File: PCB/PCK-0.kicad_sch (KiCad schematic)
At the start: 102 parts, among them J1 USB_C_Receptacle_USB2.0_16P, J2 BAT+, J3 BAT-, SW1 EN, SW10 5, SW11 M2, SW12 TAB, SW13 Q, SW14 W, SW15 E, SW16 R, SW17 T, SW18 M3, SW19 CAPSLOCK, SW2 BOOT, SW20 A, SW21 S, SW22 D, SW23 F, SW24 G, SW25 M4, SW26 LSHIFT, SW27 Z, SW28 X, SW29 C, SW3 RotaryEncoder_Switch_MP, SW30 V, SW31 SPACE, SW32 M5, SW33 FN, SW34 CTRL, SW35 SUPER, SW36 ALT, SW37 MOD1, SW38 MOD2, SW4 M1, SW5 ESC, SW6 1, SW7 2, SW8 3, SW9 4, U1 NCP1117-3.3_SOT223, U2 NCP1117-3.3_SOT223, U3 USBLC6-2SC6, U4 ESP32-C6-MINI-1, U5 TVS1400DRV

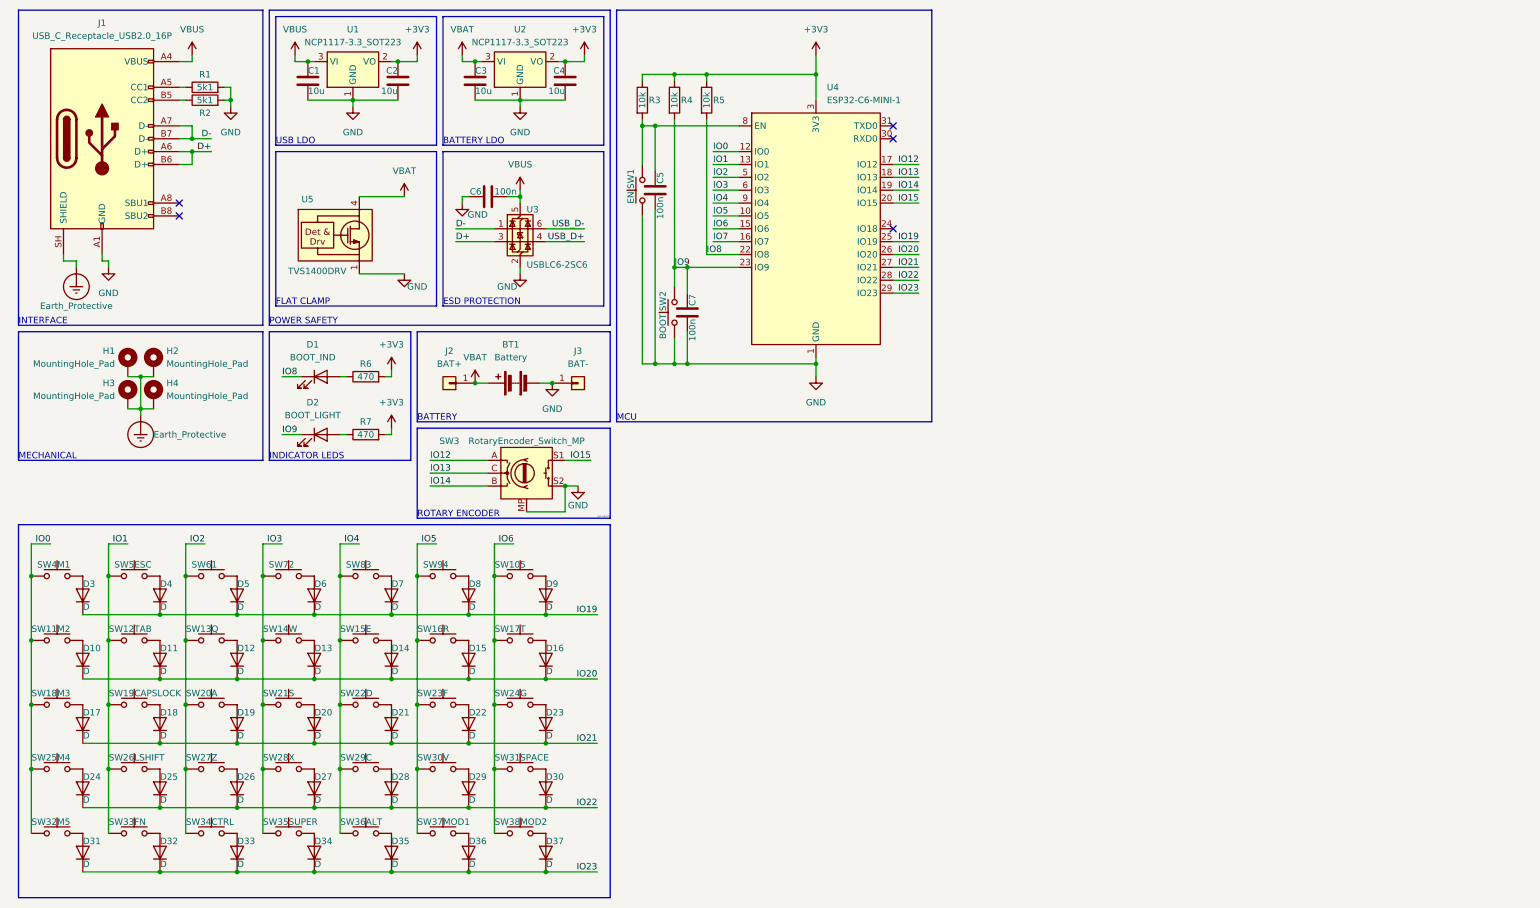
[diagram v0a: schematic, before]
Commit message: pcb start
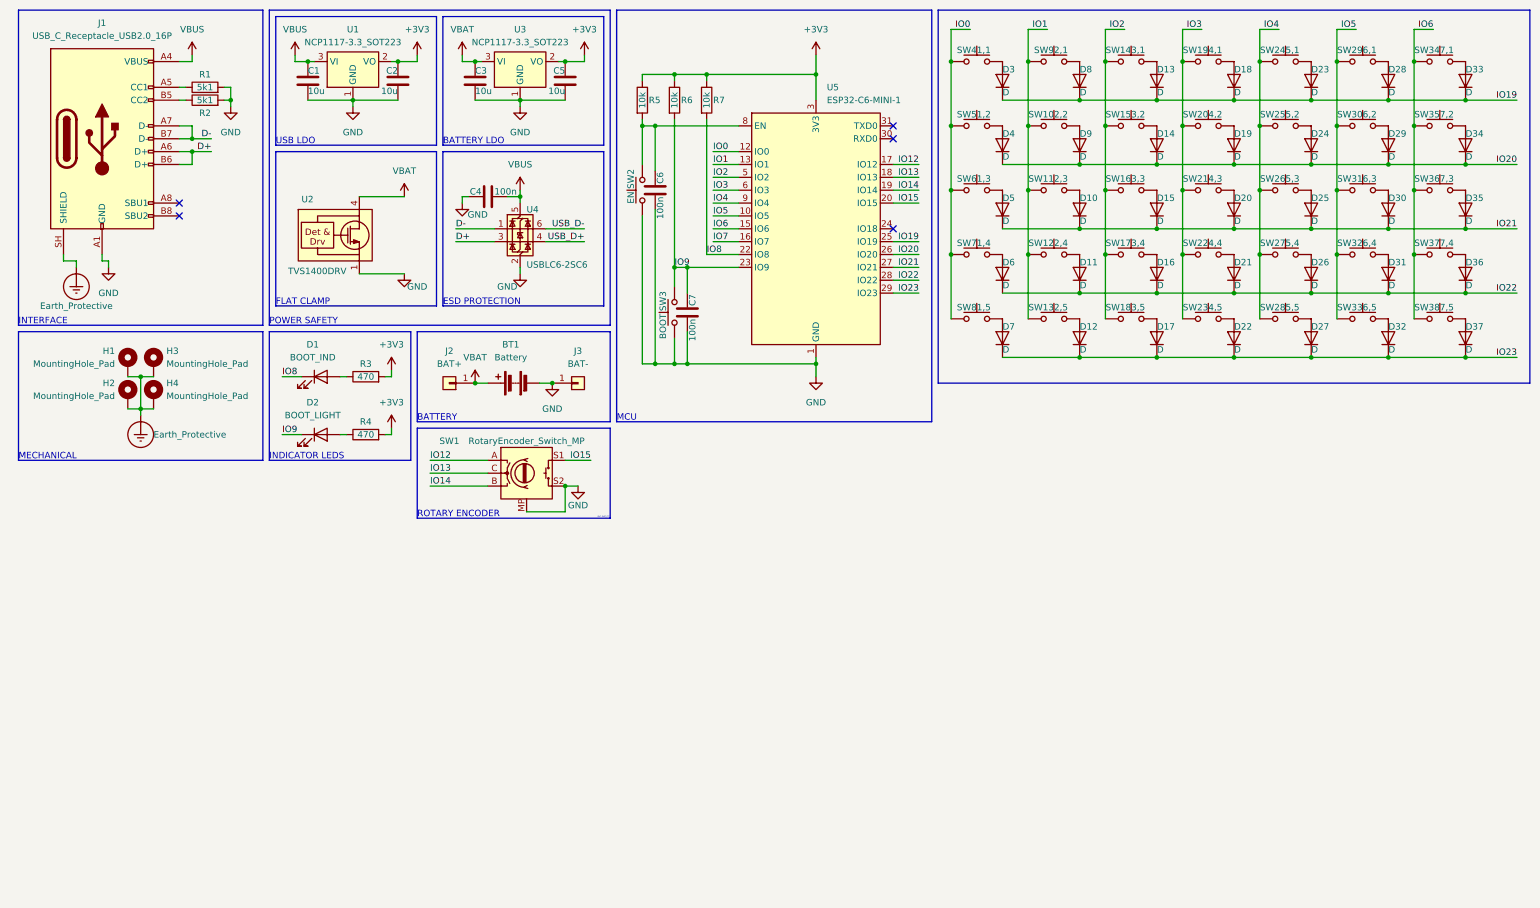
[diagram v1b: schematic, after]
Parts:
- SW10: renamed from SW12; value TAB -> 2,2
- SW11: renamed from SW19; value CAPSLOCK -> 2,3
- SW12: renamed from SW26; value LSHIFT -> 2,4
- SW13: renamed from SW33; value FN -> 2,5
- SW14: renamed from SW6; value 1 -> 3,1
- SW15: renamed from SW13; value Q -> 3,2
- SW16: renamed from SW20; value A -> 3,3
- SW17: renamed from SW27; value Z -> 3,4
- SW18: renamed from SW34; value CTRL -> 3,5
- SW19: renamed from SW7; value 2 -> 4,1
- SW20: renamed from SW14; value W -> 4,2
- SW21: value S -> 4,3
- SW22: renamed from SW28; value X -> 4,4
- SW23: renamed from SW35; value SUPER -> 4,5
- SW24: renamed from SW8; value 3 -> 5,1
- SW25: renamed from SW15; value E -> 5,2
- SW26: renamed from SW22; value D -> 5,3
- SW27: renamed from SW29; value C -> 5,4
- SW28: renamed from SW36; value ALT -> 5,5
- SW29: renamed from SW9; value 4 -> 6,1
- SW30: renamed from SW16; value R -> 6,2
- SW31: renamed from SW23; value F -> 6,3
- SW32: renamed from SW30; value V -> 6,4
- SW33: renamed from SW37; value MOD1 -> 6,5
- SW34: renamed from SW10; value 5 -> 7,1
- SW35: renamed from SW17; value T -> 7,2
- SW36: renamed from SW24; value G -> 7,3
- SW37: renamed from SW31; value SPACE -> 7,4
- SW38: value MOD2 -> 7,5
- SW4: value M1 -> 1,1
- SW5: renamed from SW11; value M2 -> 1,2
- SW6: renamed from SW18; value M3 -> 1,3
- SW7: renamed from SW25; value M4 -> 1,4
- SW8: renamed from SW32; value M5 -> 1,5
- SW9: renamed from SW5; value ESC -> 2,1
- renumbered C6 to C4, C4 to C5, C5 to C6, D18 to D10, D25 to D11, D32 to D12, D5 to D13, D12 to D14, D19 to D15, D26 to D16, D33 to D17, D6 to D18, D13 to D19, D27 to D21, D34 to D22, D7 to D23, D14 to D24, D21 to D25, D28 to D26, D35 to D27, D8 to D28, D15 to D29, D22 to D30, D29 to D31, D36 to D32, D9 to D33, D16 to D34, D23 to D35, D30 to D36, D10 to D4, D17 to D5, D24 to D6, D31 to D7, D4 to D8, D11 to D9, H3 to H2, H2 to H3, R6 to R3, R7 to R4, R3 to R5, R4 to R6, R5 to R7, SW3 to SW1, SW1 to SW2, SW2 to SW3, U5 to U2, U2 to U3, U3 to U4, U4 to U5
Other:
- moved on the sheet: D10, D11, D12, D13, D14, D15, D16, D17, D18, D19, D20, D21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
